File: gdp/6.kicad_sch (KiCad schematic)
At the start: 8 parts, among them U10 74LS83, U11 74LS244, U12 74LS244, U13 74LS244, U14 74LS244, U15 74LS244, U16 74LS244, U9 74LS83

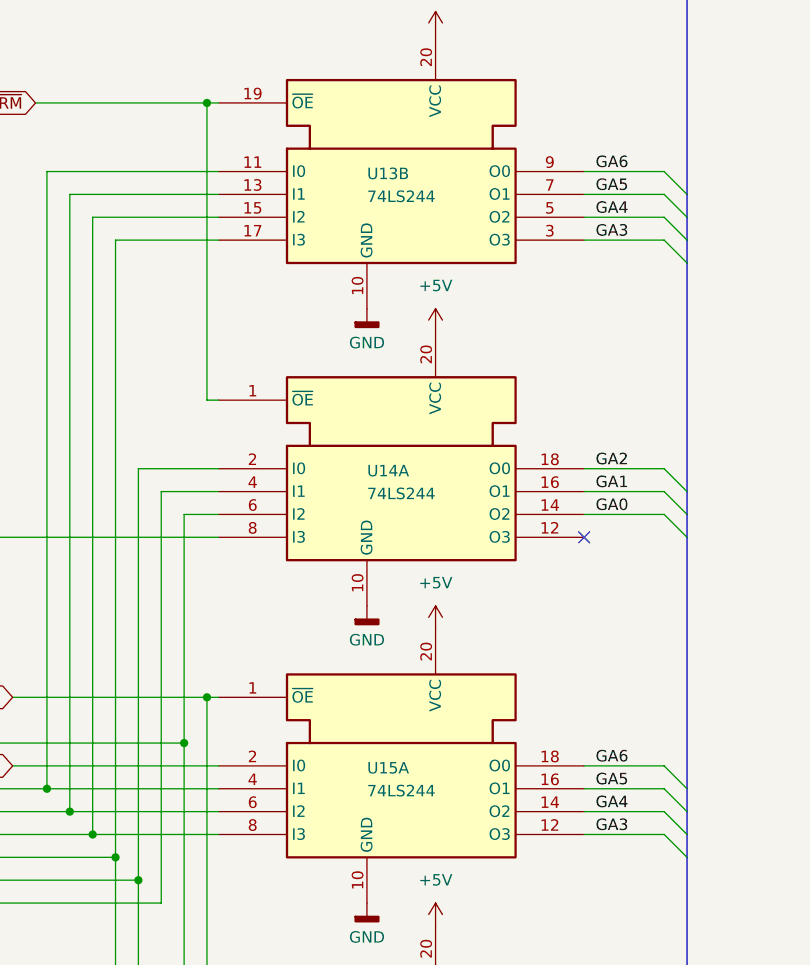
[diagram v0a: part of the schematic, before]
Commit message: Adds Sheet 8
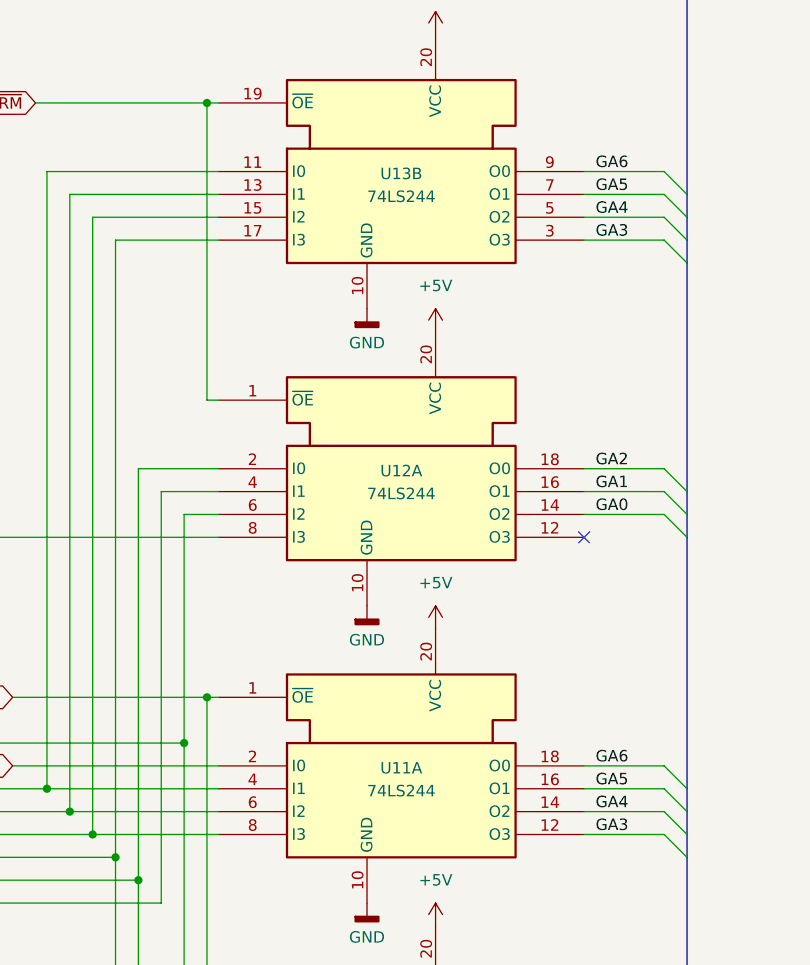
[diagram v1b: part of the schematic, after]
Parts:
- removed U14, U15: 74LS244, symbol 74xx_IEEE:74LS244
- added unit 1 of U11
- added unit 1 of U12
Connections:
- net +5V: now also U11.20 (VCC), U12.20 (VCC)
- net DAD0: now also U11.4 (I1)
- net DAD1: now also U11.6 (I2)
- net DAD2: now also U11.8 (I3)
- net DAD4: now also U12.2 (I0)
- net DAD5: now also U12.4 (I1)
- net GA0: now also U12.14 (O2)
- net GA1: now also U12.16 (O1)
- net GA2: now also U12.18 (O0)
- net GA3: now also U11.12 (O3)
- net GA4: now also U11.14 (O2)
- net GA5: now also U11.16 (O1)
- net GA6: now also U11.18 (O0)
- net GND: now also U11.10 (GND), U12.10 (GND), U12.8 (I3)
- net X9: now also U11.2 (I0)
- net ~{NORM}: now also U12.1 (~{OE})
- net ~{SHIFT}: now also U11.1 (~{OE})
- net at U10.9 (S1), U16.6 (I2): now also U12.6 (I2)
